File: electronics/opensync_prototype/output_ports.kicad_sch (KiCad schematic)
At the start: 18 parts

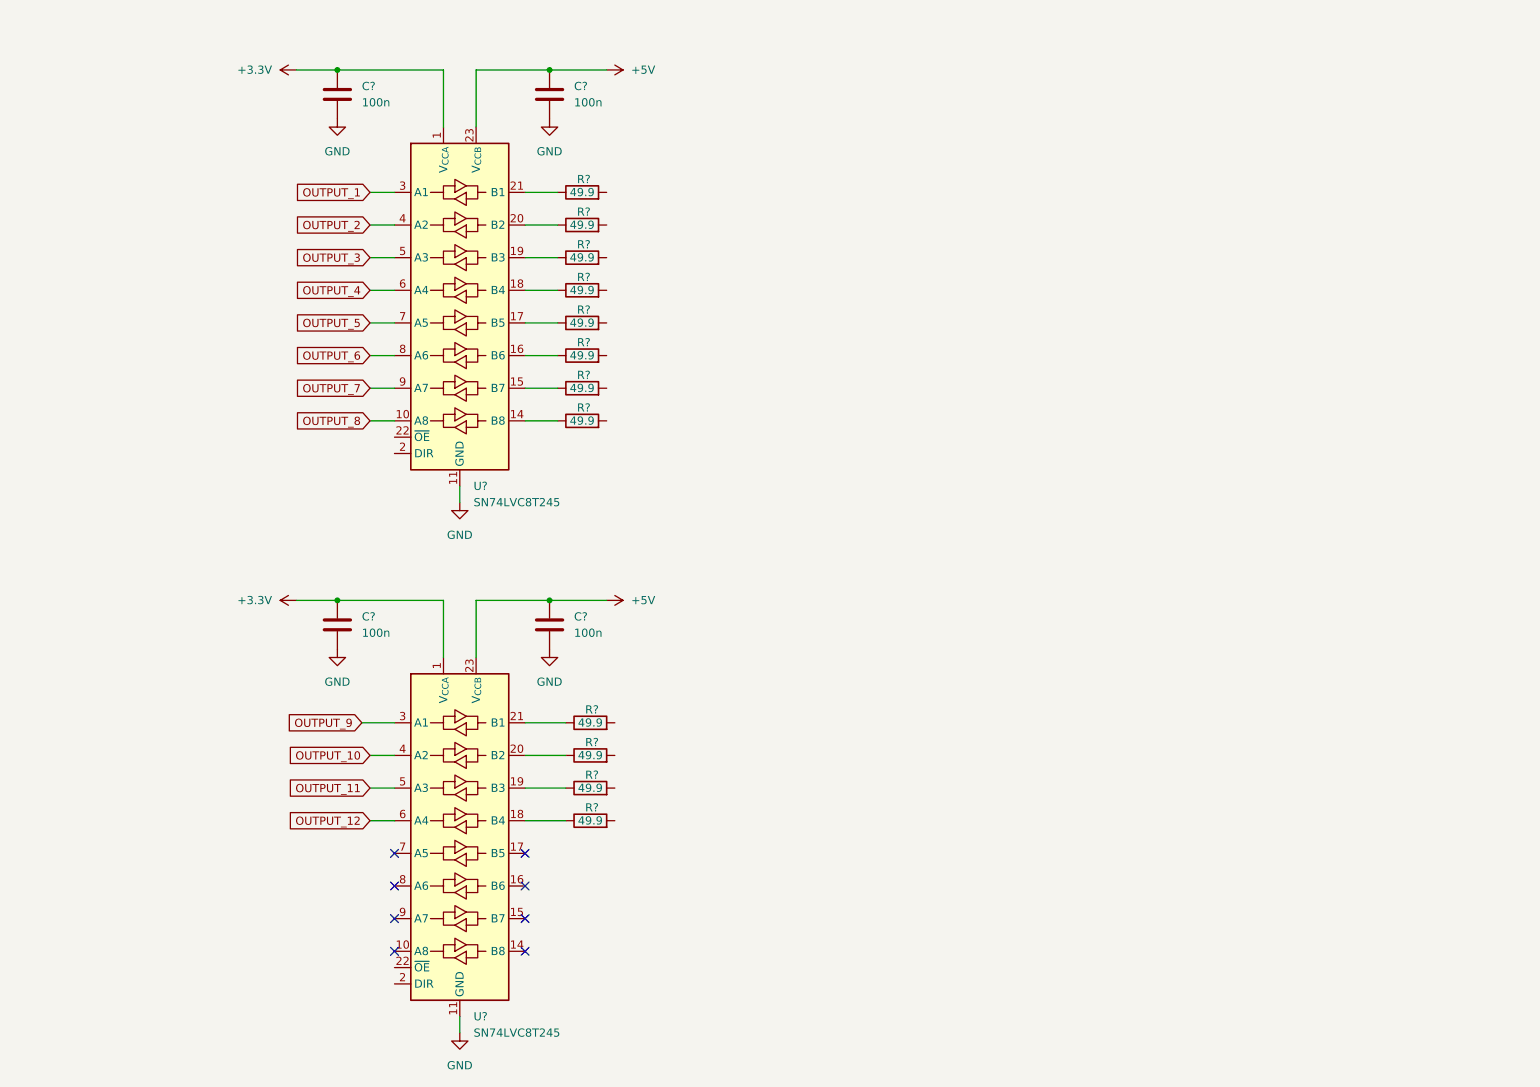
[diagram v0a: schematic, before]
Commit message: Emergency backup
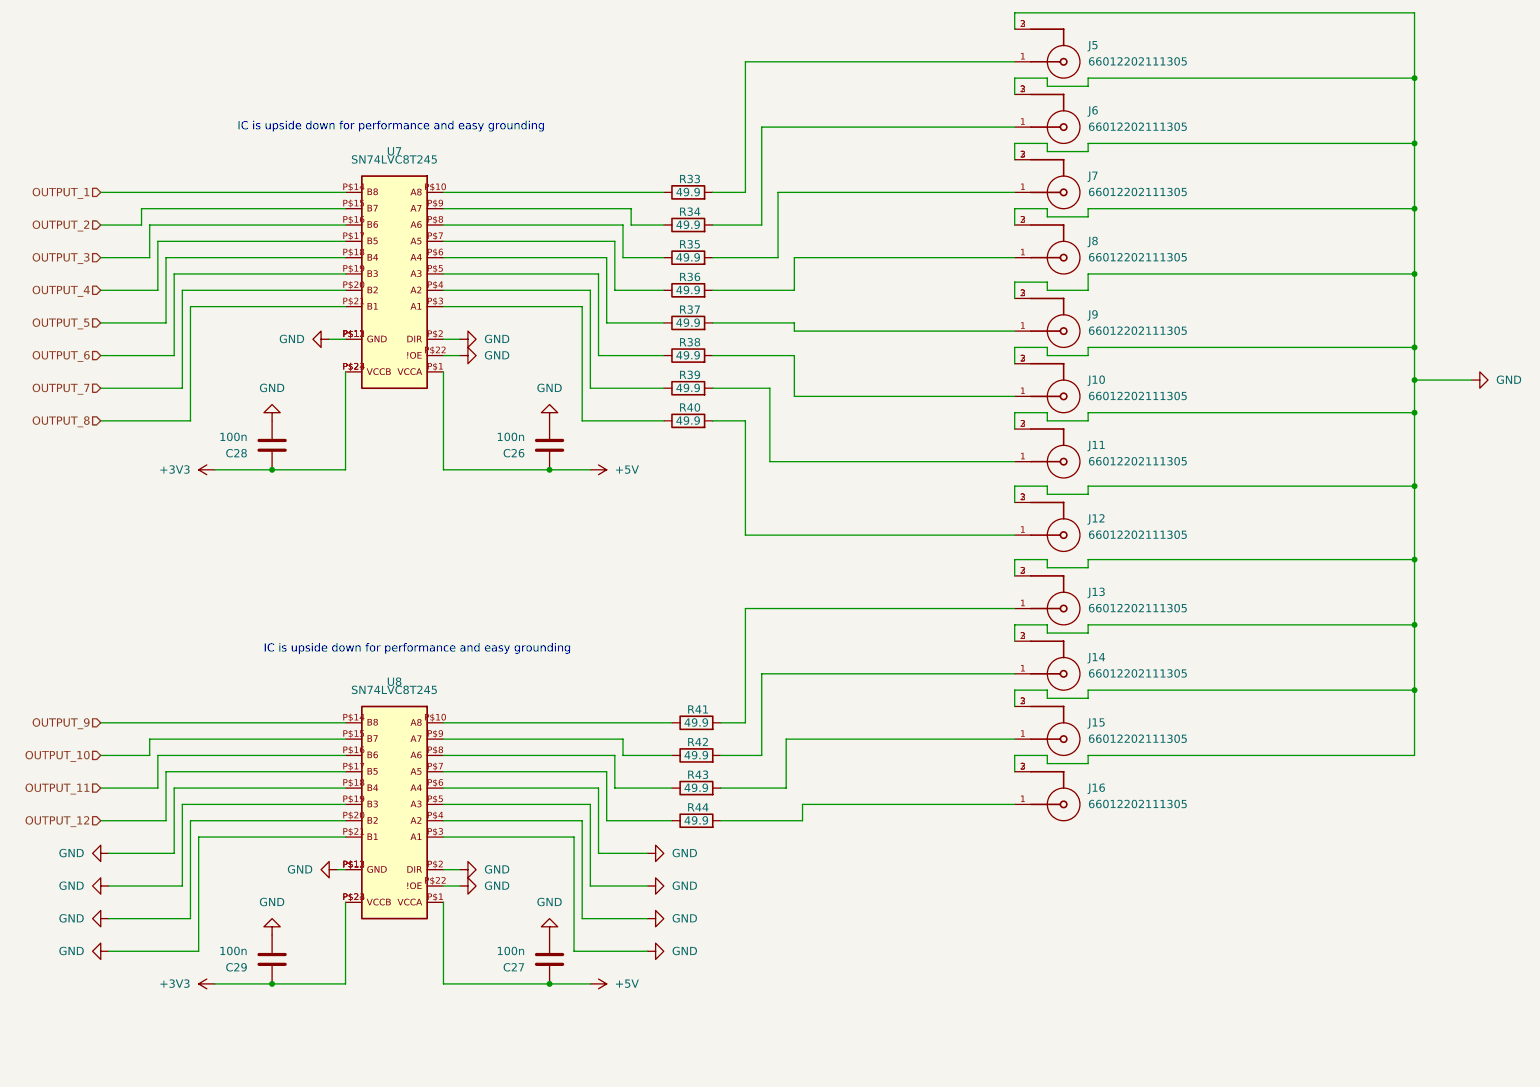
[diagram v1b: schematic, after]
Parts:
- removed U? (x2): SN74LVC8T245, symbol Logic_LevelTranslator:SN74LVC8T245
- added J10, J11, J12, J13, J14, J15, J16, J5, J6, J7, J8, J9: 66012202111305, 66012202111305:66012202111305, symbol 66012202111305:66012202111305
- added U7, U8: SN74LVC8T245, SN74LVC8T245:TTSOP-24, symbol SN74LVC8T245:SN74LVC8T245
- C26, C27, C28, C29: renamed from C?; footprint (none) -> RP2350_80QFN_minimal:C_0402_1005Metric_small_pads
- R33, R34, R35, R36, R37, R38, R39, R40, R41, R42, R43, R44: renamed from R?; footprint (none) -> Resistor_SMD:R_0402_1005Metric
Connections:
- net +3.3V is gone; now on net +5V: C26.1, C27.1
- net +5V: now also U7.P$1, U8.P$1; no longer C28.1, C29.1
- net GND: now also J10.2, J10.3, J11.2, J11.3, J12.2, J12.3, J13.2, J13.3, J14.2, J14.3, J15.2, J15.3, J16.2, J16.3, J5.2, J5.3, J6.2, J6.3, J7.2, J7.3, J8.2, J8.3, J9.2, J9.3, U7.P$11, U7.P$12, U7.P$13, U7.P$2, U7.P$22, U8.P$11, U8.P$12, U8.P$13, U8.P$18, U8.P$19, U8.P$2, U8.P$20, U8.P$21, U8.P$22, U8.P$3, U8.P$4, U8.P$5, U8.P$6
- net OUTPUT_1: now also U7.P$14
- net OUTPUT_10: now also U8.P$15
- net OUTPUT_11: now also U8.P$16
- net OUTPUT_12: now also U8.P$17
- net OUTPUT_2: now also U7.P$15
- net OUTPUT_3: now also U7.P$16
- net OUTPUT_4: now also U7.P$17
- net OUTPUT_5: now also U7.P$18
- net OUTPUT_6: now also U7.P$19
- net OUTPUT_7: now also U7.P$20
- net OUTPUT_8: now also U7.P$21
- net OUTPUT_9: now also U8.P$14
- net at R37.1: now also U7.P$6
- net at R37.2: now also J9.1
- net at R40.1: now also U7.P$3
- net at R39.1: now also U7.P$4
- net at R38.1: now also U7.P$5
- net at R36.1: now also U7.P$7
- net at R35.1: now also U7.P$8
- net at R34.1: now also U7.P$9
- net at R33.1: now also U7.P$10
- net at R35.2: now also J7.1
- net at R33.2: now also J5.1
- net at R40.2: now also J12.1
- net at R36.2: now also J8.1
- net at R44.1: now also U8.P$7
- net at R43.1: now also U8.P$8
- net at R42.1: now also U8.P$9
- net at R41.1: now also U8.P$10
- net at R41.2: now also J13.1
- net at R42.2: now also J14.1
- net at R43.2: now also J15.1
- net at R34.2: now also J6.1
- net at R39.2: now also J11.1
- net at R44.2: now also J16.1
- net at R38.2: now also J10.1
- new net +3V3: C28.1, C29.1, U7.P$23, U7.P$24, U8.P$23, U8.P$24
- no-connect marks 8 -> 0
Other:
- note added: "IC is upside down for performance and easy grounding"
- moved on the sheet: C26, C27, C28, C29, R33, R34, R35, R36, R37, R38, R39, R40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
